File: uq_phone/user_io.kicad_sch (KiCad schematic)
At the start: 26 parts, among them J7 Conn_01x02, J8 KP15B-6S-SF_800_, J9 541324562, U10 TPD3F303DQDR, U11 TPD8F003DQDR, U12 MCP1664T-E/OT, U8 LSM6DSVTR, U9 DRV2603RUNR

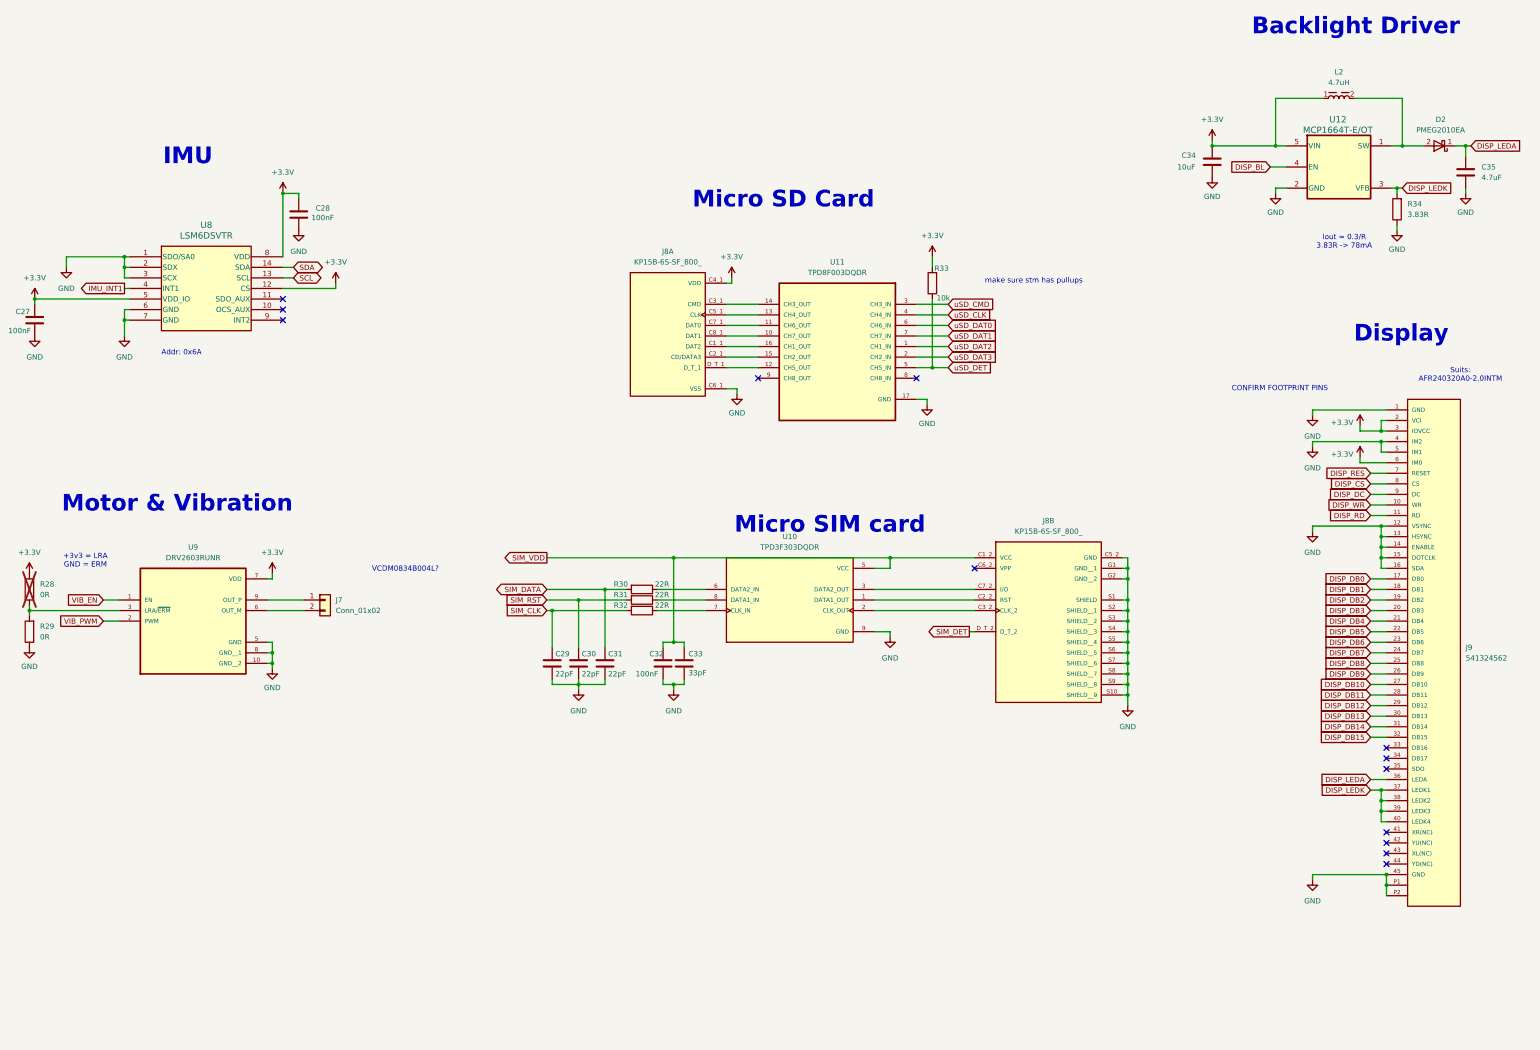
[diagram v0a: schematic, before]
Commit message: Update routing
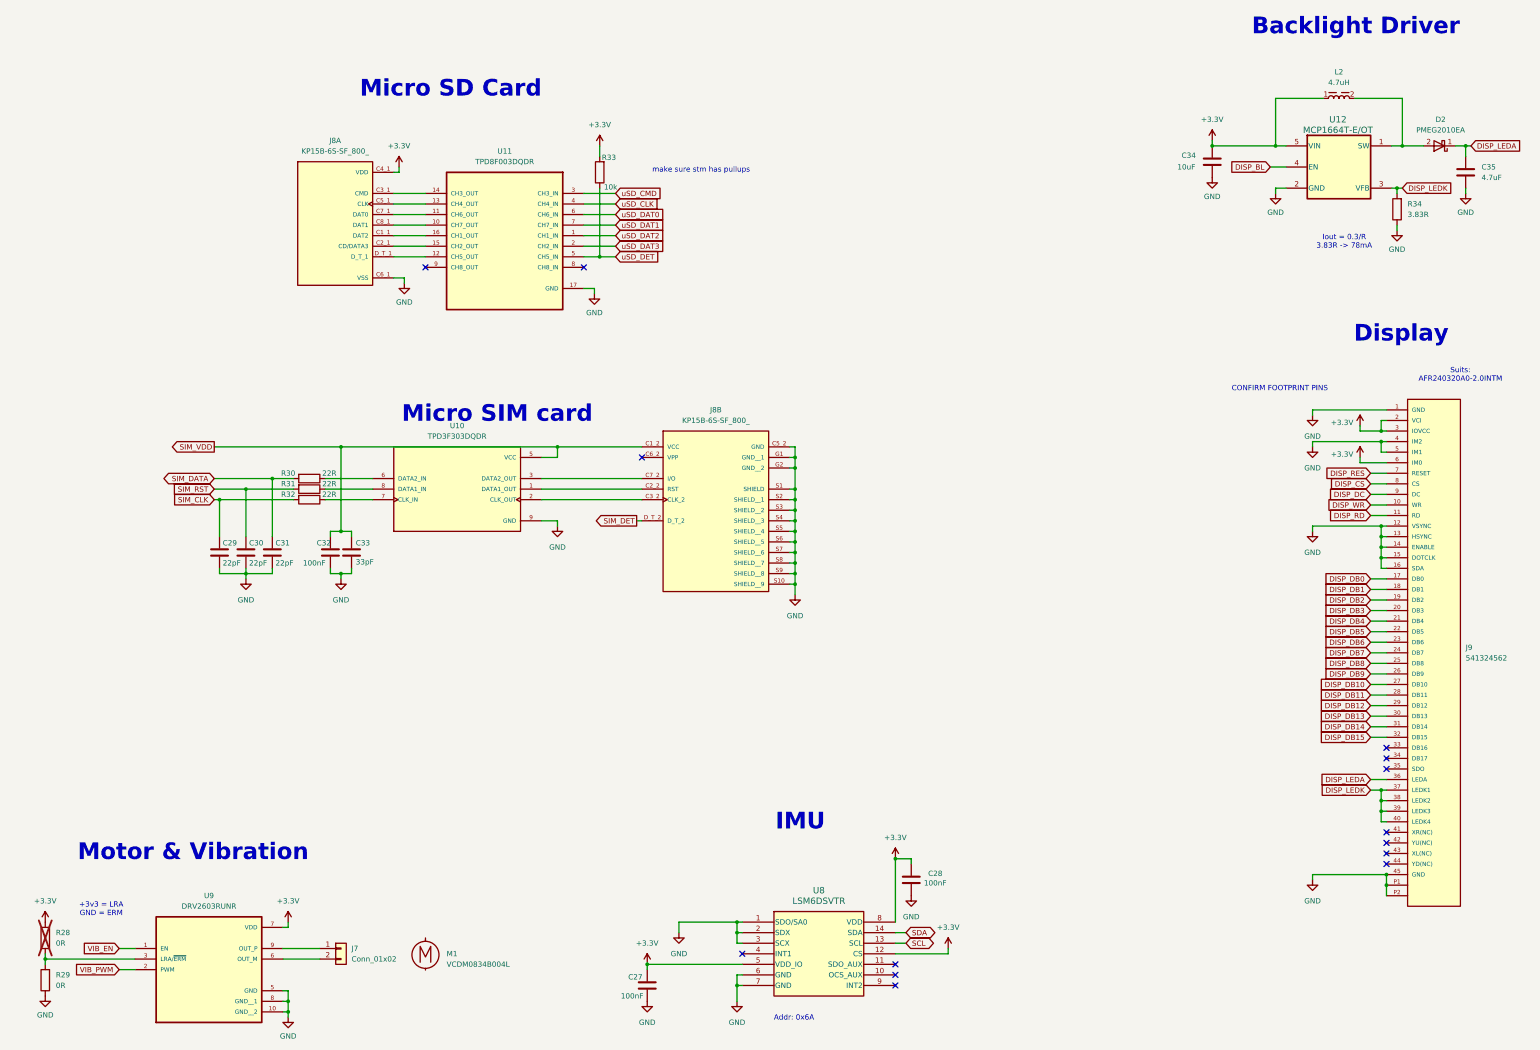
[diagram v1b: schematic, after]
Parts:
- added M1: VCDM0834B004L, custom_footprints:Motor_8mm, symbol Misc:VCDM0834B004L
- J7: footprint Connector_Wire:SolderWire-0.15sqmm_1x02_P4mm_D0.5mm_OD1.5mm -> Connector_Wire:SolderWire-0.1sqmm_1x02_P3.6mm_D0.4mm_OD1mm
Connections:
- net IMU_INT1: no longer names the net of U8.4 (INT1)
- no-connect marks 13 -> 14
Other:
- note removed: "VCDM0834B004L?"
- moved on the sheet: C27, C28, C29, C30, C31, C32, C33, J7, J8A, J8B, R28, R29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
